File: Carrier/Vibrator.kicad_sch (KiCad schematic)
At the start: 5 parts, among them M1 Z30C1T8460001, Q4 BC847

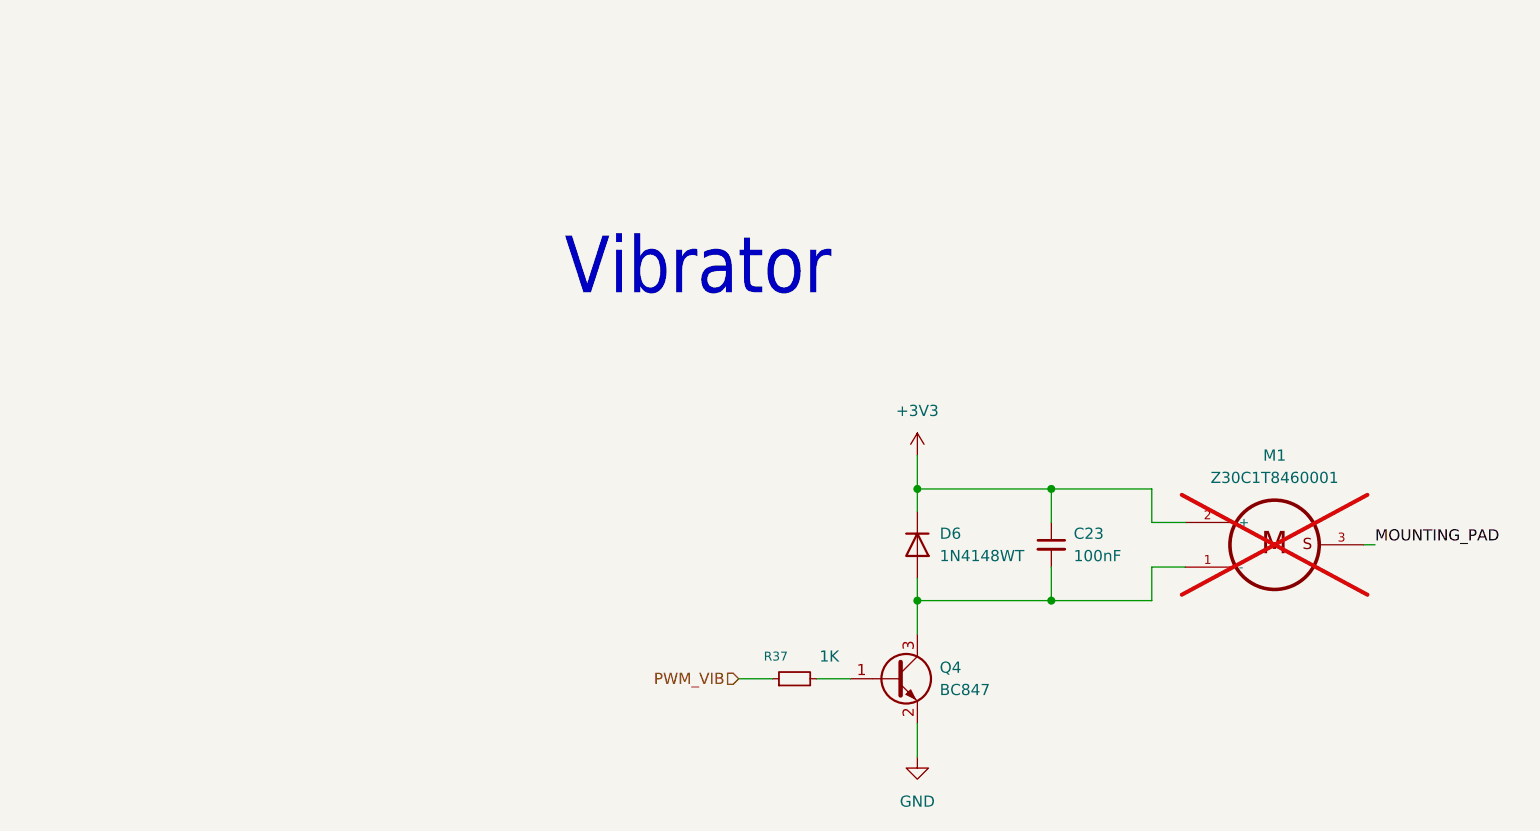
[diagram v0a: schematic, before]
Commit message: chore: lib cleanup
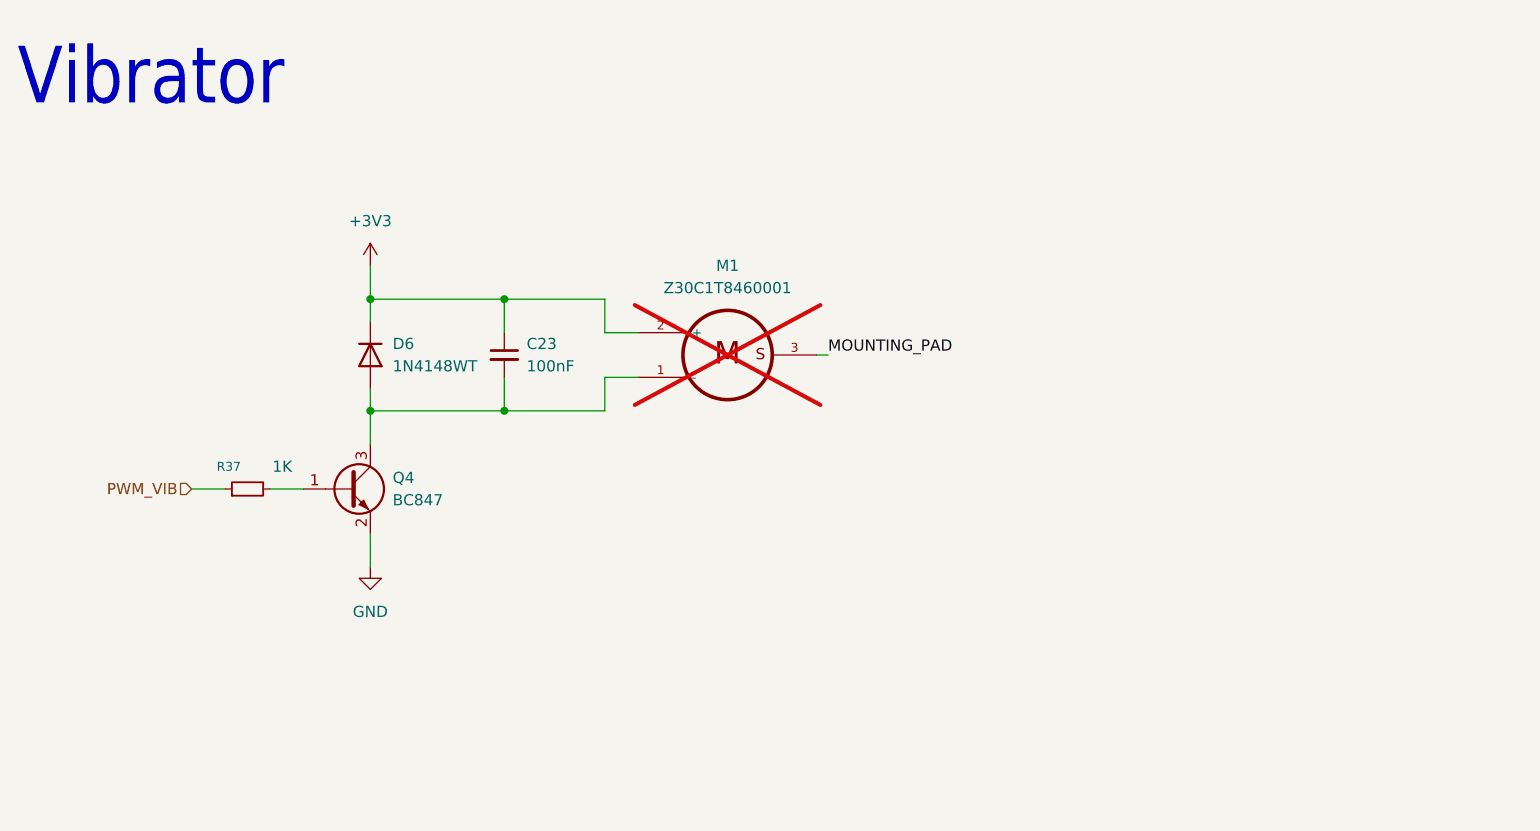
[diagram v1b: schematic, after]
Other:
- moved on the sheet: C23, D6, M1, Q4, R37
